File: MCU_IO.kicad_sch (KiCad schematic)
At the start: 34 parts, among them J8 Conn_01x02, Q1 IRLML2803, SW1 SW_Omron_B3FS, SW2 SW_Omron_B3FS, U1 MR25H40MDF, U10 USBLC6-2SC6, U11 USBLC6-2SC6, U2 RP2040, U3 MAX706RESA+, Y1 12MHz

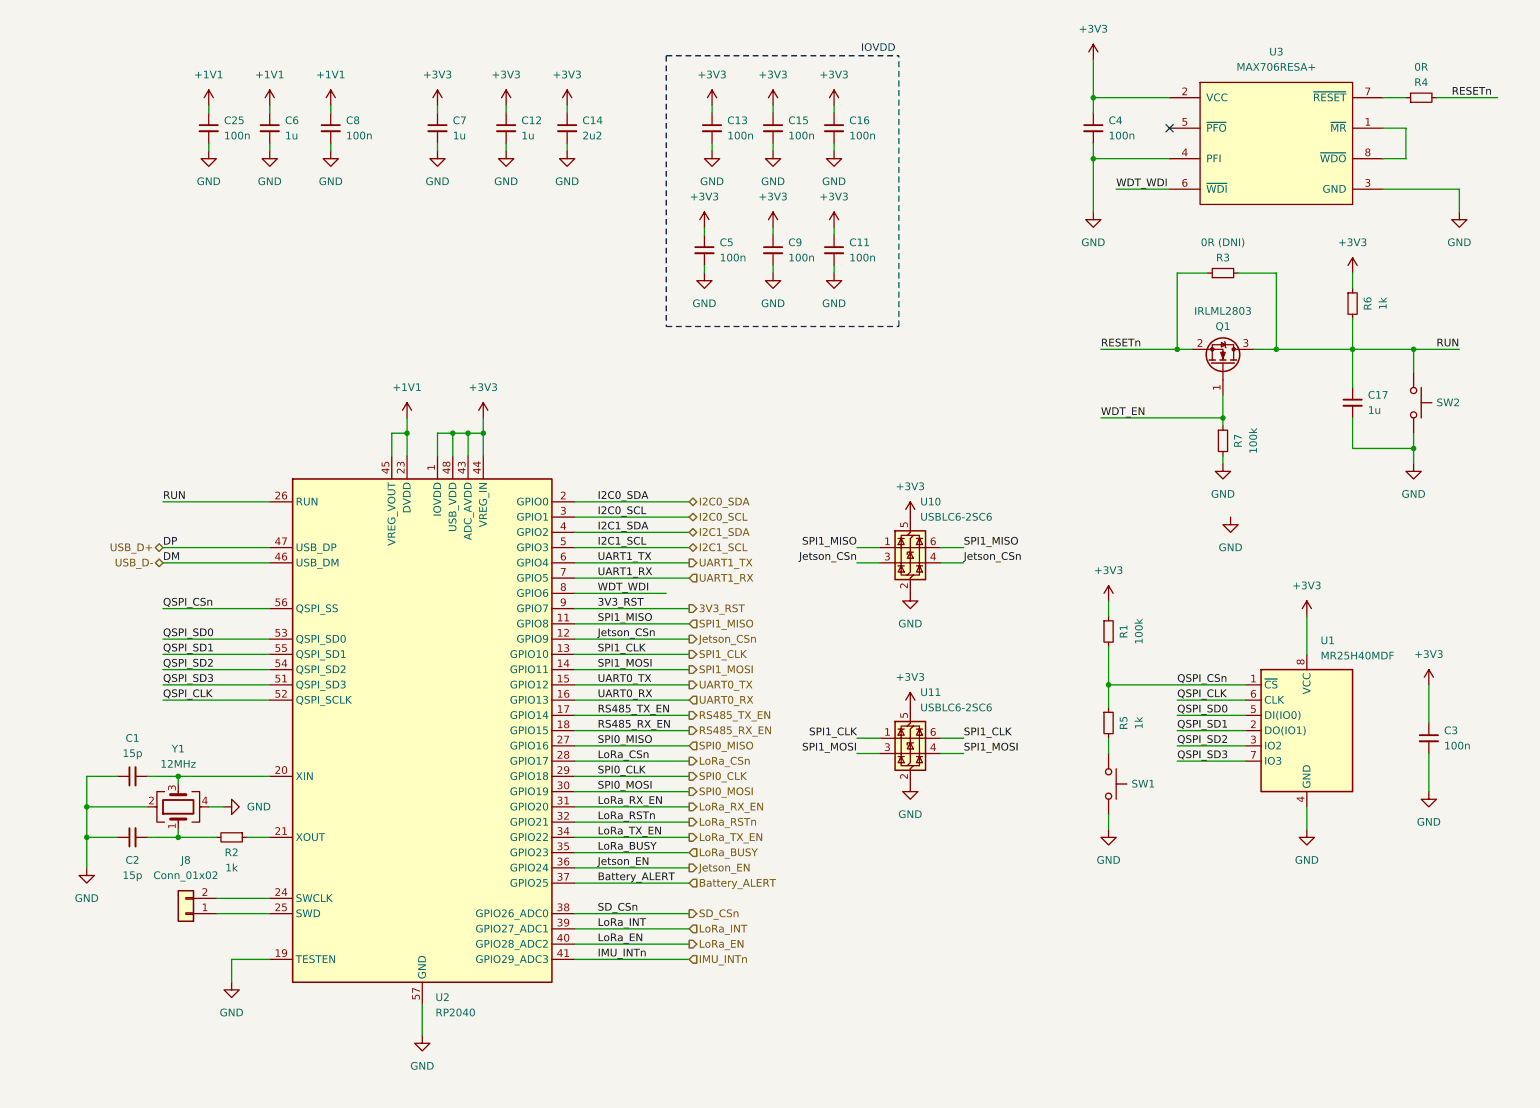
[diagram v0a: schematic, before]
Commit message: v3 partial schematic updates
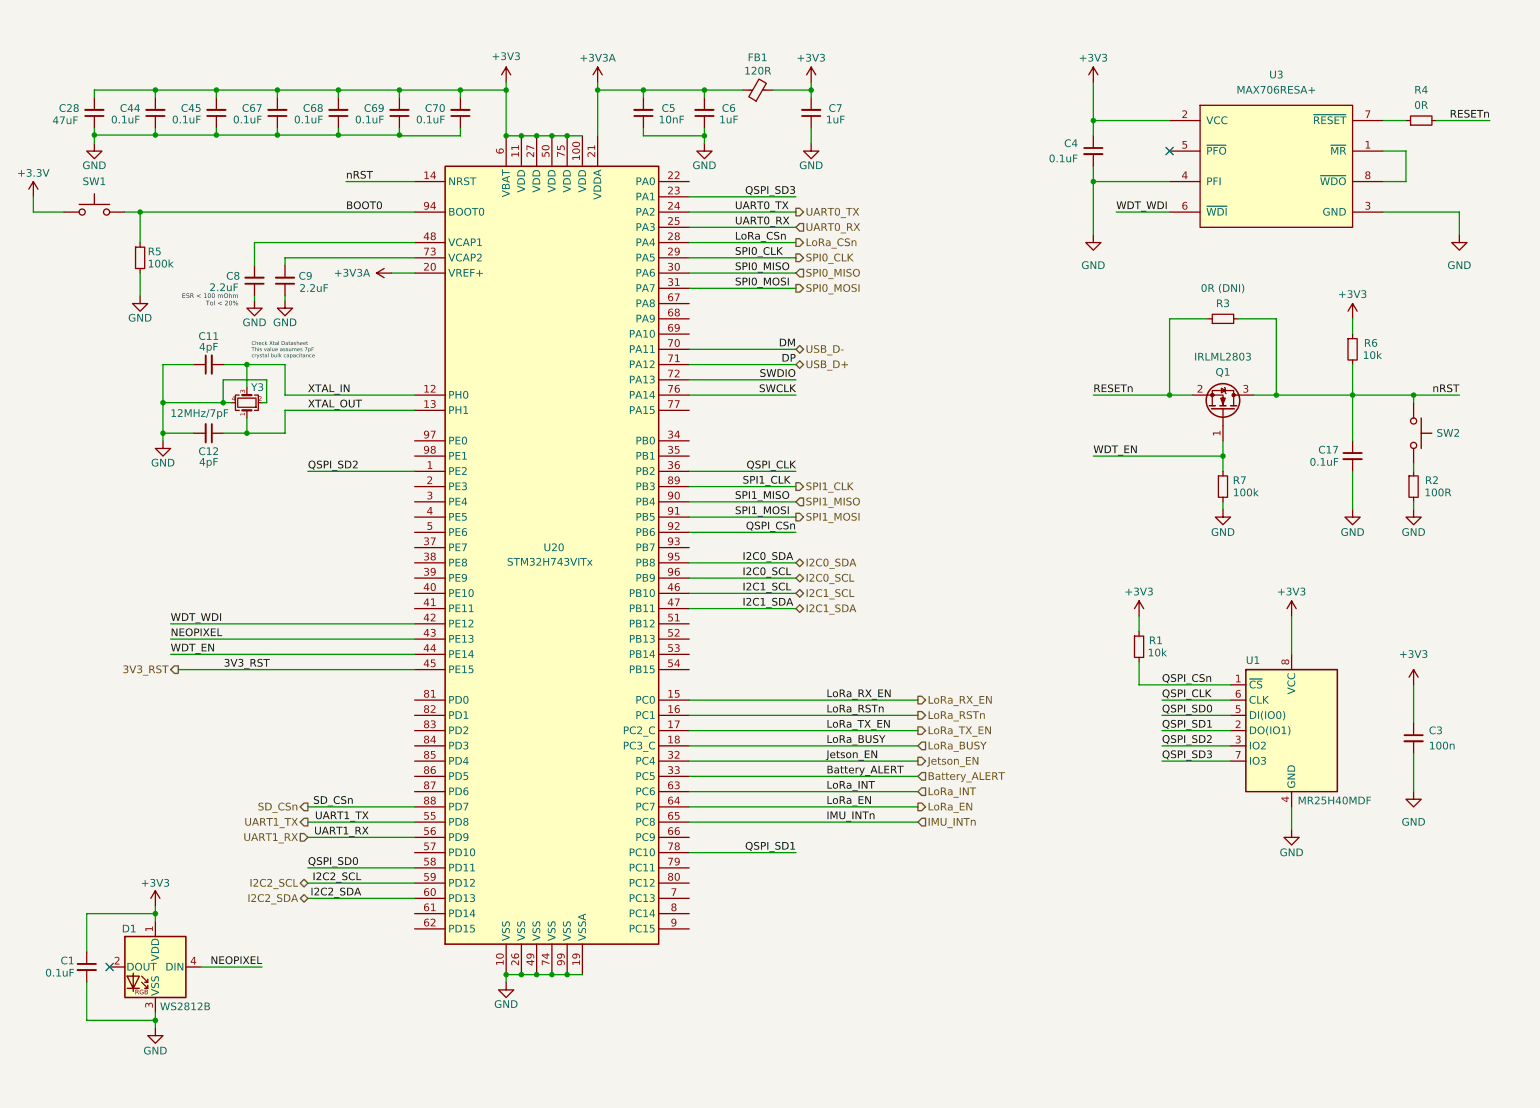
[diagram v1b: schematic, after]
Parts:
- removed C13, C15, C16, C25: 100n, Capacitor_SMD:C_0603_1608Metric, symbol Device:C_Small
- removed C14: 2u2, Capacitor_SMD:C_0603_1608Metric, symbol Device:C_Small
- removed C2: 15p, Capacitor_SMD:C_0603_1608Metric, symbol Device:C_Small
- removed J8: Conn_01x02, Connector_PinHeader_2.54mm:PinHeader_1x02_P2.54mm_Vertical, symbol Connector_Generic:Conn_01x02
- removed U10, U11: USBLC6-2SC6, Package_TO_SOT_SMD:SOT-23-6, symbol Power_Protection:USBLC6-2SC6
- removed U2: RP2040, Package_DFN_QFN:QFN-56-1EP_7x7mm_P0.4mm_EP3.2x3.2mm, symbol MCU_RaspberryPi:RP2040
- removed Y1: 12MHz, Crystal:Crystal_SMD_3225-4Pin_3.2x2.5mm, symbol Device:Crystal_GND24
- added C28: 47uF, Capacitor_SMD:C_0603_1608Metric, symbol Device:C_Small
- added C44, C45, C67, C68, C69, C70: 0.1uF, Capacitor_SMD:C_0603_1608Metric, symbol Device:C_Small
- added D1: WS2812B, LED_SMD:LED_WS2812B_PLCC4_5.0x5.0mm_P3.2mm, symbol LED:WS2812B
- added FB1: 120R, Inductor_SMD:L_0603_1608Metric, symbol Device:FerriteBead_Small
- added U20: STM32H743VITx, Package_QFP:LQFP-100_14x14mm_P0.5mm, symbol MCU_ST_STM32H7:STM32H743VITx
- added Y3: 12MHz/7pF, Crystal:Crystal_SMD_2520-4Pin_2.5x2.0mm, symbol Device:Crystal_GND24_Small
- C1: value 15p -> 0.1uF
- C11: value 100n -> 4pF
- C12: value 1u -> 4pF
- C17: value 1u -> 0.1uF
- C4: value 100n -> 0.1uF
- C5: value 100n -> 10nF
- C6, C7: value 1u -> 1uF
- C8, C9: value 100n -> 2.2uF
- R1: value 100k -> 10k
- R2: value 1k -> 100R
- R5: value 1k -> 100k; footprint Resistor_SMD:R_0603_1608Metric -> (none)
- R6: value 1k -> 10k
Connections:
- net +1V1 is gone; now on net GND: C6.1, C8.1
- net +3V3: now also C1.1, C7.2, C28.2, C44.2, C45.2, C67.2, C68.2, C69.2, C70.2, D1.1 (VDD), FB1.2, U20.100 (VDD), U20.11 (VDD), U20.27 (VDD), U20.50 (VDD), U20.6 (VBAT), U20.75 (VDD); no longer C11.1, C12.1, C5.1, C7.1, C9.1
- net 3V3_RST: now also U20.45 (PE15)
- net Battery_ALERT: now also U20.33 (PC5)
- net GND: now also C1.2, C11.1, C5.1, C7.1, C9.1, R2.2, R5.2, C28.1, C44.1, C45.1, C67.1, C68.1, C69.1, C70.1, D1.3 (VSS), U20.10 (VSS), U20.19 (VSSA), U20.26 (VSS), U20.49 (VSS), U20.74 (VSS), U20.99 (VSS), Y3.2, Y3.4; no longer C1.1, C11.2, C5.2, C6.2, C7.2, C8.2, C9.2, SW1.2, SW2.2
- net I2C0_SCL: now also U20.96 (PB9)
- net I2C0_SDA: now also U20.95 (PB8)
- net I2C1_SCL: now also U20.46 (PB10)
- net I2C1_SDA: now also U20.47 (PB11)
- net IMU_INTn: now also U20.65 (PC8)
- net Jetson_EN: now also U20.32 (PC4)
- net LoRa_BUSY: now also U20.18 (PC3_C)
- net LoRa_CSn: now also U20.28 (PA4)
- net LoRa_EN: now also U20.64 (PC7)
- net LoRa_INT: now also U20.63 (PC6)
- net LoRa_RSTn: now also U20.16 (PC1)
- net LoRa_RX_EN: now also U20.15 (PC0)
- net LoRa_TX_EN: now also U20.17 (PC2_C)
- net QSPI_CLK: now also U20.36 (PB2)
- net QSPI_CSn: now also U20.92 (PB6); no longer R5.1
- net QSPI_SD0: now also U20.58 (PD11)
- net QSPI_SD1: now also U20.78 (PC10)
- net QSPI_SD2: now also U20.1 (PE2)
- net QSPI_SD3: now also U20.23 (PA1)
- net SD_CSn: now also U20.88 (PD7)
- net SPI0_CLK: now also U20.29 (PA5)
- net SPI0_MISO: now also U20.30 (PA6)
- net SPI0_MOSI: now also U20.31 (PA7)
- net SPI1_CLK: now also U20.89 (PB3)
- net SPI1_MISO: now also U20.90 (PB4)
- net SPI1_MOSI: now also U20.91 (PB5)
- net UART0_RX: now also U20.25 (PA3)
- net UART0_TX: now also U20.24 (PA2)
- net UART1_RX: now also U20.56 (PD9)
- net UART1_TX: now also U20.55 (PD8)
- net USB_D+: now also U20.71 (PA12)
- net USB_D-: now also U20.70 (PA11)
- net WDT_EN: now also U20.44 (PE14)
- net WDT_WDI: now also U20.42 (PE12)
- net at R2.1: now also SW2.2
- net +3.3V: now reaches SW1.1
- net +3.3V: no longer R5.2
- net RUN renamed nRST
- net nRST: now also U20.14 (NRST)
- new net: C8.2, U20.48 (VCAP1)
- new net: C9.2, U20.73 (VCAP2)
- new net +3V3A: C5.2, C6.2, FB1.1, U20.20 (VREF+), U20.21 (VDDA)
- new net BOOT0: R5.1, SW1.2, U20.94 (BOOT0)
- new net I2C2_SCL: U20.59 (PD12)
- new net I2C2_SDA: U20.60 (PD13)
- new net NEOPIXEL: D1.4 (DIN), U20.43 (PE13)
- new net SWCLK: U20.76 (PA14)
- new net SWDIO: U20.72 (PA13)
- new net XTAL_IN: C11.2, U20.12 (PH0), Y3.3
- new net XTAL_OUT: C12.1, U20.13 (PH1), Y3.1
- no-connect marks 1 -> 2
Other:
- note added: "Check Xtal Datasheet This value assumes 7pF crystal bulk capacitance"
- note added: "ESR < 100 mOhm Tol < 20%"
- note removed: "IOVDD"
- moved on the sheet: C17, C3, C4, Q1, R1, R3, R4, R6, R7, SW2, U1, U3

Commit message: v3 Layout complete
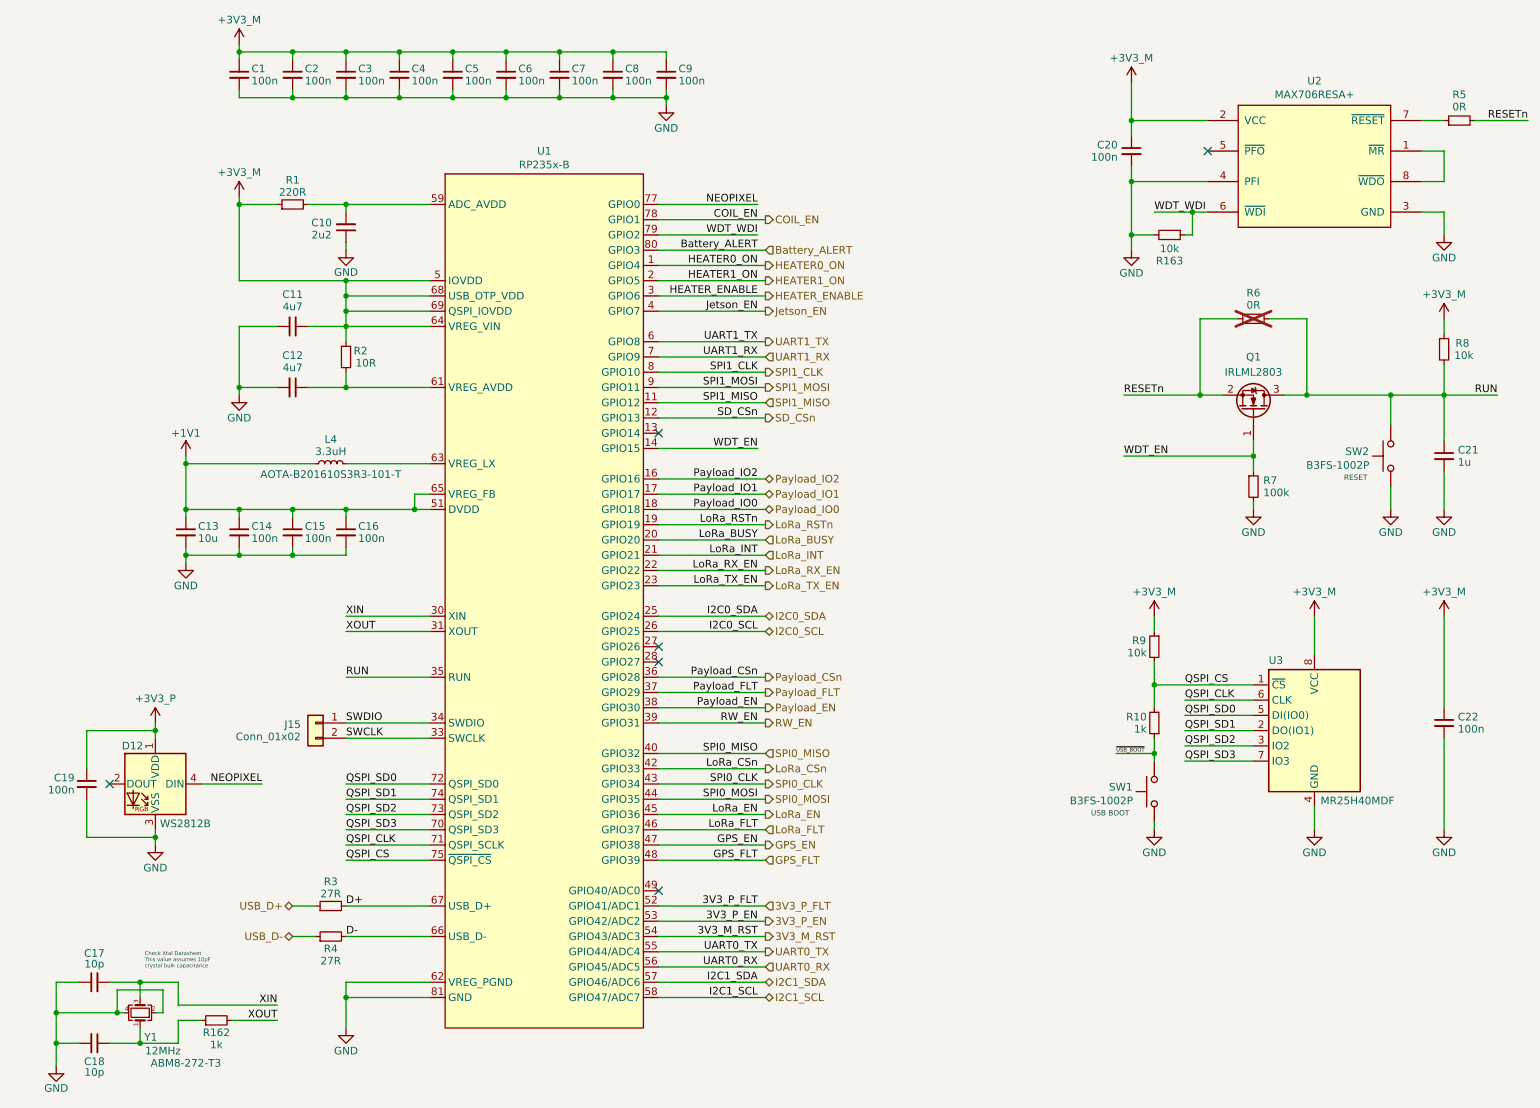
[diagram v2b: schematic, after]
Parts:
- removed C28: 47uF, Capacitor_SMD:C_0603_1608Metric, symbol Device:C_Small
- removed C44, C45, C67, C68, C69, C70: 0.1uF, Capacitor_SMD:C_0603_1608Metric, symbol Device:C_Small
- removed FB1: 120R, Inductor_SMD:L_0603_1608Metric, symbol Device:FerriteBead_Small
- removed R5: 100k, symbol Device:R_Small
- removed U20: STM32H743VITx, Package_QFP:LQFP-100_14x14mm_P0.5mm, symbol MCU_ST_STM32H7:STM32H743VITx
- removed Y3: 12MHz/7pF, Crystal:Crystal_SMD_2520-4Pin_2.5x2.0mm, symbol Device:Crystal_GND24_Small
- added C1, C14, C15, C16, C2, C3, C4: 100n, Capacitor_SMD:C_0603_1608Metric, symbol Device:C_Small
- added C10: 2u2, Capacitor_SMD:C_0603_1608Metric, symbol Device:C_Small
- added C13: 10u, Capacitor_SMD:C_0805_2012Metric, symbol Device:C_Small
- added C17, C18: 10p, Capacitor_SMD:C_0603_1608Metric, symbol Device:C_Small
- added J15: Conn_01x02, Connector_PinHeader_2.54mm:PinHeader_1x02_P2.54mm_Vertical, symbol Connector_Generic:Conn_01x02
- added L4: 3.3uH, Argus-Passives:L_0806_2016Metric, symbol Device:L_Small
- added R1: 220R, Resistor_SMD:R_0603_1608Metric, symbol Device:R_Small
- added R10, R162: 1k, Resistor_SMD:R_0603_1608Metric, symbol Device:R_Small
- added R163: 10k, Resistor_SMD:R_0603_1608Metric, symbol Device:R_Small
- added R3, R4: 27R, Resistor_SMD:R_0603_1608Metric, symbol Device:R_Small
- added U1: RP235x-B, Argus-IC:RP2350-QFN-80-1EP_10x10_P0.4mm_EP3.4x3.4mm_ThermalVias, symbol Argus-IC:RP235x-B
- added Y1: 12MHz, Crystal:Crystal_SMD_3225-4Pin_3.2x2.5mm, symbol Device:Crystal_GND24_Small
- C11, C12: value 4pF -> 4u7; footprint Capacitor_SMD:C_0603_1608Metric -> Capacitor_SMD:C_0805_2012Metric
- C19: renamed from C1; value 0.1uF -> 100n
- C20: renamed from C4; value 0.1uF -> 100n
- C21: renamed from C17; value 0.1uF -> 1u
- C5: value 10nF -> 100n
- C6, C7: value 1uF -> 100n
- C8, C9: value 2.2uF -> 100n
- Q1: symbol MainBoard:IRLML2803 -> Argus-IC:IRLML2803
- R2: value 100R -> 10R
- R6: renamed from R3; value 0R (DNI) -> 0R; now not fitted
- SW1, SW2: value SW_Omron_B3FS -> B3FS-1002P; footprint Button_Switch_SMD:SW_SPST_Omron_B3FS-105xP -> Button_Switch_SMD:SW_SPST_B3U-1000P
- U3: renamed from U1; symbol Memory_Flash:W25Q32JVSS -> Argus-IC:FLASH_QSPI
- renumbered C3 to C22, D1 to D12, R4 to R5, R6 to R8, R1 to R9, U3 to U2
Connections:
- net +3.3V is gone; now on net GND: SW1.1
- net +3V3A is gone; now on net GND: C5.2, C6.2
- net XTAL_IN is gone; now on net +3V3_M: C11.2
- net Battery_ALERT: now also U1.80 (GPIO3)
- net GND: now also C7.2, C8.2, C9.2, SW2.1, U3.9 (GND), C1.2, C10.1, C13.2, C14.2, C15.2, C16.2, C17.1, C18.2, C2.2, C3.2, C4.2, R163.2, U1.62 (VREG_PGND), U1.81 (GND), Y1.2, Y1.4; no longer C5.1, C6.1, C7.1, C8.1, C9.1, R2.2
- net I2C0_SCL: now also U1.26 (GPIO25)
- net I2C0_SDA: now also U1.25 (GPIO24)
- net I2C1_SCL: now also U1.58 (GPIO47/ADC7)
- net I2C1_SDA: now also U1.57 (GPIO46/ADC6)
- net Jetson_EN: now also U1.4 (GPIO7)
- net LoRa_BUSY: now also U1.20 (GPIO20)
- net LoRa_CSn: now also U1.42 (GPIO33)
- net LoRa_EN: now also U1.45 (GPIO36)
- net LoRa_INT: now also U1.21 (GPIO21)
- net LoRa_RSTn: now also U1.19 (GPIO19)
- net LoRa_RX_EN: now also U1.22 (GPIO22)
- net LoRa_TX_EN: now also U1.23 (GPIO23)
- net NEOPIXEL: now also U1.77 (GPIO0)
- net QSPI_CLK: now also U1.71 (QSPI_SCLK)
- net QSPI_SD0: now also U1.72 (QSPI_SD0)
- net QSPI_SD1: now also U1.74 (QSPI_SD1)
- net QSPI_SD2: now also U1.73 (QSPI_SD2)
- net QSPI_SD3: now also U1.70 (QSPI_SD3)
- net SD_CSn: now also U1.12 (GPIO13)
- net SPI0_CLK: now also U1.43 (GPIO34)
- net SPI0_MISO: now also U1.40 (GPIO32)
- net SPI0_MOSI: now also U1.44 (GPIO35)
- net SPI1_CLK: now also U1.8 (GPIO10)
- net SPI1_MISO: now also U1.11 (GPIO12)
- net SPI1_MOSI: now also U1.9 (GPIO11)
- net SWCLK: now also J15.2 (Pin_2), U1.33 (SWCLK)
- net SWDIO: now also J15.1 (Pin_1), U1.34 (SWDIO)
- net UART0_RX: now also U1.56 (GPIO45/ADC5)
- net UART0_TX: now also U1.55 (GPIO44/ADC4)
- net UART1_RX: now also U1.7 (GPIO9)
- net UART1_TX: now also U1.6 (GPIO8)
- net USB_D+: now also R3.1
- net USB_D-: now also R4.1
- net WDT_EN: now also U1.14 (GPIO15)
- net WDT_WDI: now also R163.1, U1.79 (GPIO2)
- net +3V3_M: now reaches R2.1
- net +3V3_M: now also C20.1, C22.1, C5.1, C6.1, C7.1, C8.1, C9.1, R8.1, R9.1, U2.2 (VCC), U3.8 (VCC), C1.1, C2.1, C3.1, C4.1, R1.1, U1.15 (IOVDD), U1.24 (IOVDD), U1.29 (IOVDD), U1.41 (IOVDD), U1.5 (IOVDD), U1.50 (IOVDD), U1.60 (IOVDD), U1.64 (VREG_VIN), U1.68 (USB_OTP_VDD), U1.69 (QSPI_IOVDD), U1.76 (IOVDD); no longer SW2.2
- removed net +3V3: C19.1, C20.1, C22.1, C7.2, D12.1 (VDD), R8.1, R9.1, U2.2 (VCC), U3.8 (VCC)
- net BOOT0 renamed ~{USB_BOOT}
- net ~{USB_BOOT}: now also R10.1
- net QSPI_CSn renamed QSPI_CS
- net QSPI_CS: now also R10.2, U1.75 (~{QSPI_CS})
- net XTAL_OUT: no longer names the net of C12.1
- net XTAL_OUT: now also R2.2, U1.61 (VREG_AVDD)
- net nRST renamed RUN
- net RUN: now also SW2.2, U1.35 (RUN); no longer SW2.1
- new net: C10.2, R1.2, U1.59 (ADC_AVDD)
- new net: L4.2, U1.63 (VREG_LX)
- new net: C18.1, R162.1, Y1.1
- new net +1V1: C13.1, C14.1, C15.1, C16.1, L4.1, U1.10 (DVDD), U1.32 (DVDD), U1.51 (DVDD), U1.65 (VREG_FB)
- new net +3V3_P: C19.1, D12.1 (VDD)
- new net 3V3_M_RST: U1.54 (GPIO43/ADC3)
- new net 3V3_P_EN: U1.53 (GPIO42/ADC2)
- new net 3V3_P_FLT: U1.52 (GPIO41/ADC1)
- new net COIL_EN: U1.78 (GPIO1)
- new net D+: R3.2, U1.67 (USB_D+)
- new net D-: R4.2, U1.66 (USB_D-)
- new net GPS_EN: U1.47 (GPIO38)
- new net GPS_FLT: U1.48 (GPIO39)
- new net HEATER0_ON: U1.1 (GPIO4)
- new net HEATER1_ON: U1.2 (GPIO5)
- new net HEATER_ENABLE: U1.3 (GPIO6)
- new net LoRa_FLT: U1.46 (GPIO37)
- new net Payload_CSn: U1.36 (GPIO28)
- new net Payload_EN: U1.38 (GPIO30)
- new net Payload_FLT: U1.37 (GPIO29)
- new net Payload_IO0: U1.18 (GPIO18)
- new net Payload_IO1: U1.17 (GPIO17)
- new net Payload_IO2: U1.16 (GPIO16)
- new net RW_EN: U1.39 (GPIO31)
- new net XIN: C17.2, U1.30 (XIN), Y1.3
- new net XOUT: R162.2, U1.31 (XOUT)
- no-connect marks 2 -> 6
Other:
- note added: "Check Xtal Datasheet This value assumes 10pF crystal bulk capacitance"
- note added: "RESET"
- note added: "USB BOOT"
- note removed: "Check Xtal Datasheet This value assumes 7pF crystal bulk capacitance"
- note removed: "ESR < 100 mOhm Tol < 20%"
- moved on the sheet: C19, C20, C21, C22, D12, Q1, R5, R7, R8, R9, U2, U3
